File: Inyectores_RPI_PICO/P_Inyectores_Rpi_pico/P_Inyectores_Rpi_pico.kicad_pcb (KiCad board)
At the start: 2 copper layers, 127 x 139 mm, 98 parts, among them J1 Entrada_12V/4A, J2 Conn_01x07_Male, K1 SANYOU_SRD_Form_C, K2 SANYOU_SRD_Form_C, Q1 IRF540N, Q2 IRF540N, Q3 IRF540N, Q4 IRF540N, Q5 BC548, Q6 BC548, Q7 BC548, SW1 PUSH2, SW2 Reset_Push, SW3 Rotary_Encoder_Switch, SW4 PUSH1, U1 PC817, U10 DS3231M, U11 AT24CS32-XHM, U2 PC817, U3 PC817, U4 PC817, U5 L7805, U6 AMS1117-3.3, U7 Pico, U8 PC817, U9 PC817

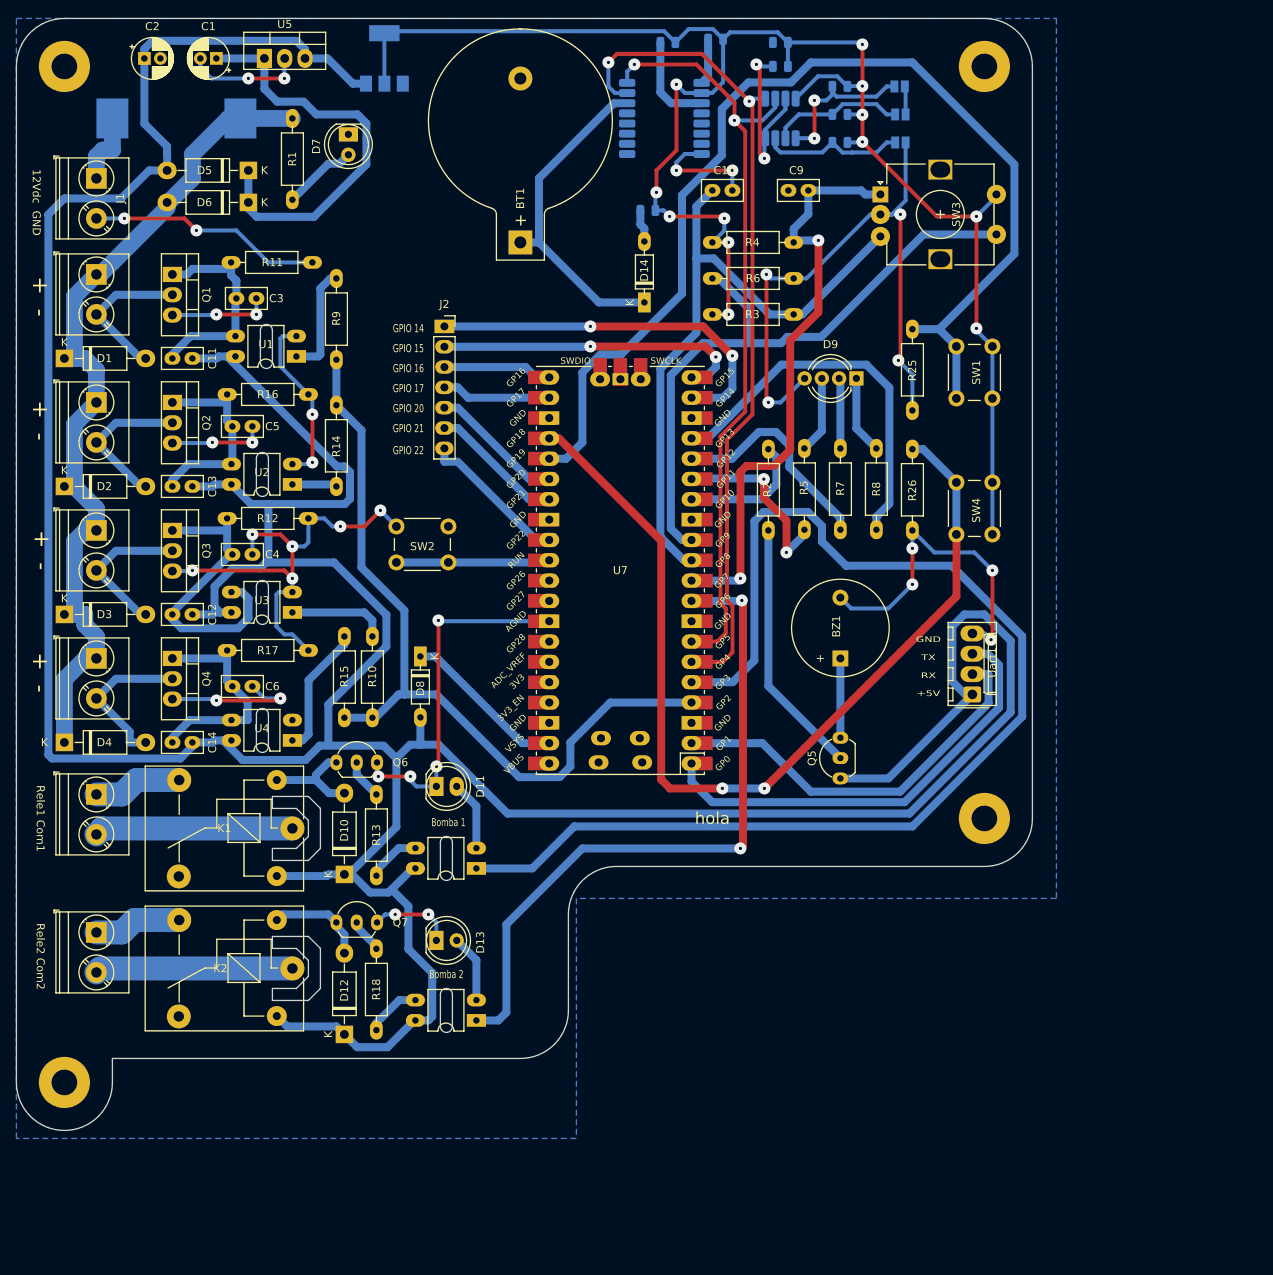
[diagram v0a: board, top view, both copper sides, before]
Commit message: Insoladora UV
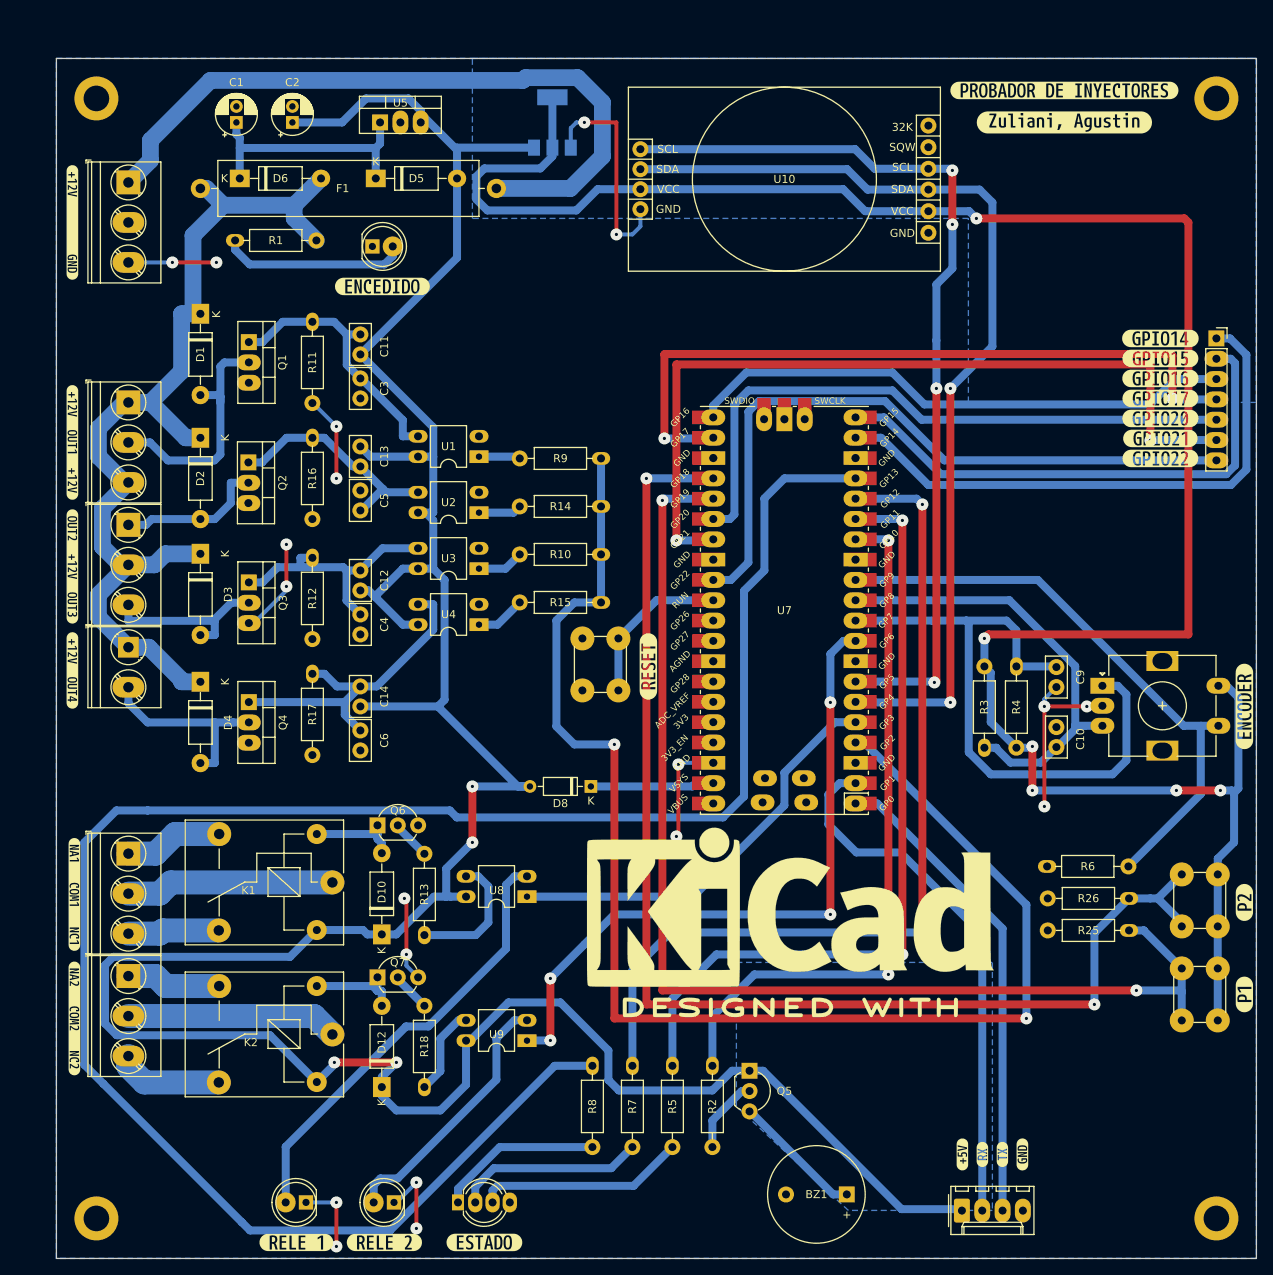
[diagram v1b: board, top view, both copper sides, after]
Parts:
- removed BT1: Battery_Cell, Battery:BatteryHolder_Keystone_103_1x20mm
- removed Bornera_rele1, Bornera_rele2, SAL_INY1, SAL_INY2, SAL_INY3: Screw_Terminal_01x02, Bornera_Tornillos:TerminalBlock_Phoenix_PT-1,5-2-5.0-H_1x02_P5.00mm_Horizontal
- removed C7, C8: 0.1uf, Capacitor_SMD:C_0805_2012Metric
- removed D14: 1N4148, Diode_THT:D_DO-35_SOD27_P7.62mm_Horizontal
- removed JP1: A0, Jumper:SolderJumper-2_P1.3mm_Open_Pad1.0x1.5mm
- removed JP2: A1, Jumper:SolderJumper-2_P1.3mm_Open_Pad1.0x1.5mm
- removed JP3: A2, Jumper:SolderJumper-2_P1.3mm_Open_Pad1.0x1.5mm
- removed R19: 200 1/8W 5%, Resistor_SMD:R_0805_2012Metric
- removed R20, R21: 4K7 1/8W 5%, Resistor_SMD:R_0805_2012Metric
- removed R22, R23, R24: 10k, Resistor_SMD:R_0805_2012Metric
- removed Tornillo1, Tornillo2, Tornillo3, Tornillo4: MountingHole_3.2mm_M3_Pad, MountingHole:MountingHole_3.2mm_M3_Pad
- removed U11: AT24CS32-XHM, Package_SO:SOIC-8_3.9x4.9mm_P1.27mm
- added ?: , , F.Cu at (170.0, 30.0)
- added J3: B1_INY, Borneras:TerminalBlock_Phoenix_PT-1,5-3-5.0-H_1x03_P5.00mm_Horizontal, F.Cu at (34.0, 68.0)
- added J4: BOR2_INY, Borneras:TerminalBlock_Phoenix_PT-1,5-3-5.0-H_1x03_P5.00mm_Horizontal, F.Cu at (34.0, 83.3)
- added J5: BOR1_RELE, Borneras:TerminalBlock_Phoenix_PT-1,5-3-5.0-H_1x03_P5.00mm_Horizontal, F.Cu at (34.0, 124.4)
- added J6: BOR2_RELE, Borneras:TerminalBlock_Phoenix_PT-1,5-3-5.0-H_1x03_P5.00mm_Horizontal, F.Cu at (34.0, 139.7)
- added REF3: MountingHole_3.2mm_M3_ISO14580_Pad, MountingHole:MountingHole_3.2mm_M3_ISO14580_Pad, F.Cu at (30.0, 170.0)
- added REF4: MountingHole_3.2mm_M3_ISO14580_Pad, MountingHole:MountingHole_3.2mm_M3_ISO14580_Pad, F.Cu at (170.0, 170.0)
- added REF5: MountingHole_3.2mm_M3_ISO14580_Pad, MountingHole:MountingHole_3.2mm_M3_ISO14580_Pad, F.Cu at (30.0, 30.0)
- added kibuzzard-62C09447: G***, kibuzzard-62C09447, F.Cu at (151.0, 33.0)
- added kibuzzard-62C09473: G***, kibuzzard-62C09473, F.Cu at (151.0, 29.0)
- added kibuzzard-62C095A2: G***, kibuzzard-62C095A2, F.Cu at (163.0, 60.0)
- added kibuzzard-62C095AC: G***, kibuzzard-62C095AC, F.Cu at (163.0, 62.5)
- added kibuzzard-62C095B6: G***, kibuzzard-62C095B6, F.Cu at (163.0, 65.0)
- added kibuzzard-62C095BF: G***, kibuzzard-62C095BF, F.Cu at (163.0, 67.5)
- added kibuzzard-62C095C6: G***, kibuzzard-62C095C6, F.Cu at (163.0, 70.0)
- added kibuzzard-62C095D0: G***, kibuzzard-62C095D0, F.Cu at (163.0, 72.5)
- added kibuzzard-62C095D9: G***, kibuzzard-62C095D9, F.Cu at (163.0, 75.0)
- added kibuzzard-62C09649: G***, kibuzzard-62C09649, F.Cu at (173.5, 142.0)
- added kibuzzard-62C09656: G***, kibuzzard-62C09656, F.Cu at (173.5, 130.5)
- added kibuzzard-62C09664: G***, kibuzzard-62C09664, F.Cu at (173.5, 106.0)
- added kibuzzard-62C0966F: G***, kibuzzard-62C0966F, F.Cu at (99.0, 101.0)
- added kibuzzard-62C096C0: G***, kibuzzard-62C096C0, F.Cu at (55.0, 173.0)
- added kibuzzard-62C096D5: G***, kibuzzard-62C096D5, F.Cu at (66.0, 173.0)
- added kibuzzard-62C096DE: G***, kibuzzard-62C096DE, F.Cu at (78.5, 173.0)
- added kibuzzard-62C096F9: G***, kibuzzard-62C096F9, F.Cu at (65.8, 53.5)
- added kibuzzard-62C09818: G***, kibuzzard-62C09818, F.Cu at (27.0, 88.5)
- added kibuzzard-62C09846: G***, kibuzzard-62C09846, F.Cu at (27.0, 101.5)
- added kibuzzard-62C098BB: G***, kibuzzard-62C098BB, F.Cu at (27.0, 73.0)
- added kibuzzard-62C09983: G***, kibuzzard-62C09983, F.Cu at (138.2, 162.0)
- added kibuzzard-62C099B8: G***, kibuzzard-62C099B8, F.Cu at (140.8, 162.0)
- added kibuzzard-62C099BF: G***, kibuzzard-62C099BF, F.Cu at (143.2, 162.0)
- added kibuzzard-62C099C8: G***, kibuzzard-62C099C8, F.Cu at (145.8, 162.0)
- added kibuzzard-62C099DD: G***, kibuzzard-62C099DD, F.Cu at (27.0, 45.5)
- added kibuzzard-62C09A4A: G***, kibuzzard-62C09A4A, F.Cu at (27.2, 129.5)
- added kibuzzard-62C09A65: G***, kibuzzard-62C09A65, F.Cu at (27.2, 145.0)
- F1: footprint Bornera_Tornillos:Fuse_20x5mm -> Fuse:Fuse_SunFuse-6HP; moved to F.Cu
- J1: footprint Bornera_Tornillos:TerminalBlock_Phoenix_PT-1,5-2-5.0-H_1x02_P5.00mm_Horizontal -> Borneras:TerminalBlock_Phoenix_PT-1,5-3-5.0-H_1x03_P5.00mm_Horizontal
- REF1: moved to F.Cu
- SAL_INY4: value Screw_Terminal_01x02 -> BOR3_INY; footprint Bornera_Tornillos:TerminalBlock_Phoenix_PT-1,5-2-5.0-H_1x02_P5.00mm_Horizontal -> Borneras:TerminalBlock_Phoenix_PT-1,5-2-5.0-H_1x02_P5.00mm_Horizontal
- U10: value DS3231M -> DS3231_SHIELD; footprint Package_SO:SOIC-16W_7.5x10.3mm_P1.27mm -> DS3231_SHIELD:DS3231_Shield; moved to F.Cu
- moved D9 114.4 mm to (75.2, 168.0), turned to 0 degrees
- moved J2 96.5 mm to (170.0, 60.0)
- moved R8 94.3 mm to (92.0, 161.1), turned to 90 degrees
- moved R7 91.1 mm to (97.0, 161.1), turned to 90 degrees
- moved R6 90.0 mm to (159.0, 126.0), turned to 180 degrees
- moved R5 88.9 mm to (102.0, 161.1), turned to 90 degrees
- moved SW1 82.7 mm to (170.2, 138.8)
- moved C10 81.8 mm to (150.0, 111.1), turned to 90 degrees
- moved R2 77.4 mm to (107.0, 161.1)
- moved R4 73.7 mm to (145.0, 111.2), turned to 90 degrees
- moved SW3 67.4 mm to (155.8, 103.4)
- moved R25 67.2 mm to (148.9, 134.0), turned to 0 degrees
- moved C9 67.2 mm to (150.0, 101.1), turned to -90 degrees
- moved BZ1 67.0 mm to (123.8, 167.0), turned to 180 degrees
- moved Uart1 64.5 mm to (138.2, 169.0), turned to 0 degrees
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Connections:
- net Net-(D1-Pad2) renamed /Control/INY1_OUT
- net Net-(D2-Pad2) renamed /Control/INY2_OUT
- net Net-(D3-Pad2) renamed /Control/INY3_OUT
- J1 pad 2: GND -> unconnected-(J1-Pad2)
- K1 pad 3: /Control/Sal_Rele1 -> /Control/Sal1_Rele1
- K1 pad 4: Net-(K1-Pad4) -> /Control/Sal2_Rele1
- K2 pad 3: /Control/Sal_Rele2 -> /Control/Sal1_Rele2
- K2 pad 4: Net-(K2-Pad4) -> /Control/Sal2_Rele2
- U10 pad 1: Net-(R20-Pad2) -> /Control/I2C0_SCL
- U10 pad 2: +3V3 -> /Control/I2C0_SDA
- U10 pad 3: Net-(R21-Pad2) -> +3V3
- U10 pad 4: Net-(U10-Pad4) -> GND
- U10 pad 5: GND -> unconnected-(U10-Pad5)
- U10 pad 6: GND -> unconnected-(U10-Pad6)
- U7 pad 13: Net-(U7-Pad13) -> unconnected-(U7-Pad13)
- U7 pad 18: Net-(U7-Pad18) -> unconnected-(U7-Pad18)
- U7 pad 23: Net-(U7-Pad23) -> unconnected-(U7-Pad23)
- U7 pad 28: Net-(U7-Pad28) -> unconnected-(U7-Pad28)
- U7 pad 3: Net-(U7-Pad3) -> unconnected-(U7-Pad3)
- U7 pad 31: Net-(U7-Pad31) -> unconnected-(U7-Pad31)
- U7 pad 32: Net-(U7-Pad32) -> unconnected-(U7-Pad32)
- U7 pad 34: Net-(U7-Pad34) -> unconnected-(U7-Pad34)
- U7 pad 35: Net-(U7-Pad35) -> unconnected-(U7-Pad35)
- U7 pad 36: Net-(U7-Pad36) -> unconnected-(U7-Pad36)
- U7 pad 37: Net-(U7-Pad37) -> unconnected-(U7-Pad37)
- U7 pad 40: Net-(U7-Pad40) -> unconnected-(U7-Pad40)
- U7 pad 41: Net-(U7-Pad41) -> unconnected-(U7-Pad41)
- U7 pad 42: Net-(U7-Pad42) -> unconnected-(U7-Pad42)
- U7 pad 43: Net-(U7-Pad43) -> unconnected-(U7-Pad43)
- U7 pad 8: Net-(U7-Pad8) -> unconnected-(U7-Pad8)
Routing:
- net GND: track 382.4 -> 127.7 mm, vias 36 -> 19
- net /Control/Rgb3: track 48.2 -> 244.7 mm
- net +5V: track 507.5 -> 391.2 mm, vias 0 -> 4
- net /Control/Bomba1: track 154.1 -> 52.5 mm
- net /Control/GPIO21: track 16.8 -> 103.7 mm, vias 0 -> 2
- net /Control/Rgb2: track 27.5 -> 112.5 mm, vias 0 -> 2
- net Net-(F1-Pad2): track 9.03 -> 89.1 mm
- net /Control/GPIO17: track 13.6 -> 91.2 mm, vias 0 -> 2
- net /Control/Rgb1: track 23.2 -> 99.6 mm
- net /Control/INYECTORES: track 99.9 -> 175.7 mm, vias 0 -> 2
- net /Control/Buzzer: track 16.2 -> 88.8 mm, vias 0 -> 2
- net +3V3: track 215.1 -> 283.2 mm, vias 12 -> 6
- net /Control/GPIO22: track 18.8 -> 86.3 mm
- net /Control/GPIO20: track 16.8 -> 79.1 mm
- net /Control/GPIO16: track 13.6 -> 69.1 mm
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- added copper zone on B.Cu, net +3V3
- added copper zone on B.Cu, net +5V
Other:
- board size 127 x 139 mm -> 150 x 150 mm
- board text removed: "+ -"
- board text removed: "12Vdc GND"
- board text removed: "Bomba 1"
- board text removed: "Bomba 2"
- board text removed: "GND TX RX +5V"
- board text removed: "GPIO 14"
- board text removed: "GPIO 15"
- board text removed: "GPIO 16"
- board text removed: "GPIO 17"
- board text removed: "GPIO 20"
- board text removed: "GPIO 21"
- board text removed: "GPIO 22"
- board text removed: "Rele1 Com1"
- board text removed: "Rele2 Com2"
- board text removed: "Zuliani, Agustin"
- board text removed: "hola"

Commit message: .
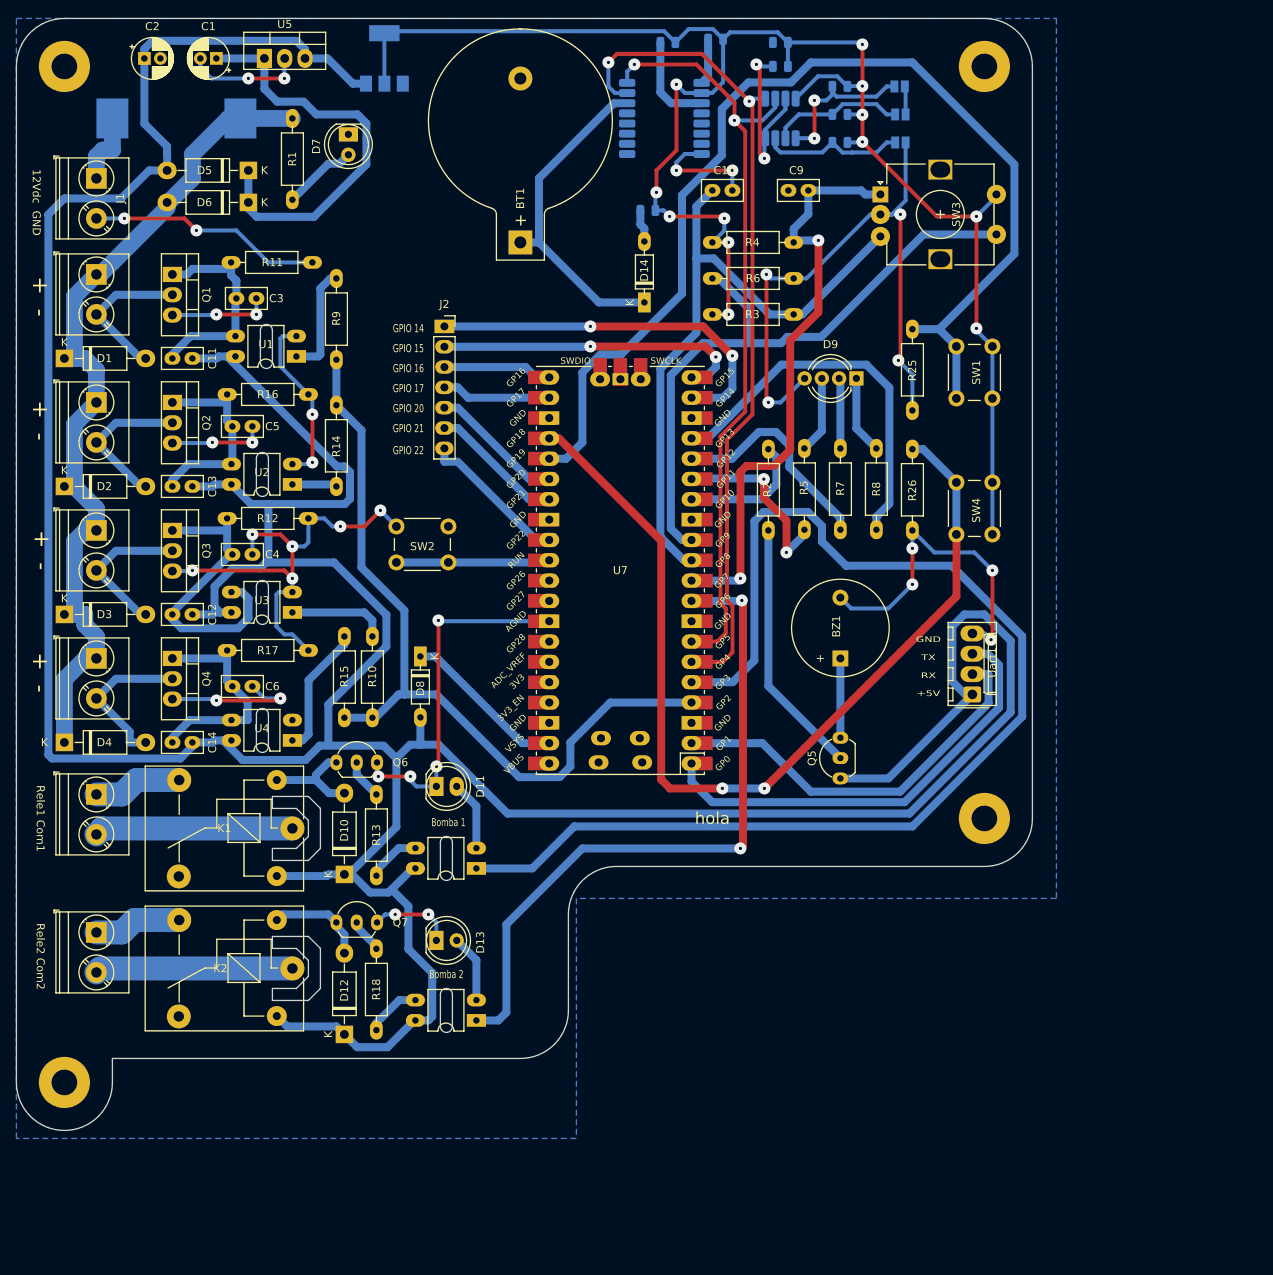
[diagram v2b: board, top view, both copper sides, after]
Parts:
- removed ?: , 
- removed J3: B1_INY, Borneras:TerminalBlock_Phoenix_PT-1,5-3-5.0-H_1x03_P5.00mm_Horizontal
- removed J4: BOR2_INY, Borneras:TerminalBlock_Phoenix_PT-1,5-3-5.0-H_1x03_P5.00mm_Horizontal
- removed J5: BOR1_RELE, Borneras:TerminalBlock_Phoenix_PT-1,5-3-5.0-H_1x03_P5.00mm_Horizontal
- removed J6: BOR2_RELE, Borneras:TerminalBlock_Phoenix_PT-1,5-3-5.0-H_1x03_P5.00mm_Horizontal
- removed REF3, REF4, REF5: MountingHole_3.2mm_M3_ISO14580_Pad, MountingHole:MountingHole_3.2mm_M3_ISO14580_Pad
- removed kibuzzard-62C09447: G***, kibuzzard-62C09447
- removed kibuzzard-62C09473: G***, kibuzzard-62C09473
- removed kibuzzard-62C095A2: G***, kibuzzard-62C095A2
- removed kibuzzard-62C095AC: G***, kibuzzard-62C095AC
- removed kibuzzard-62C095B6: G***, kibuzzard-62C095B6
- removed kibuzzard-62C095BF: G***, kibuzzard-62C095BF
- removed kibuzzard-62C095C6: G***, kibuzzard-62C095C6
- removed kibuzzard-62C095D0: G***, kibuzzard-62C095D0
- removed kibuzzard-62C095D9: G***, kibuzzard-62C095D9
- removed kibuzzard-62C09649: G***, kibuzzard-62C09649
- removed kibuzzard-62C09656: G***, kibuzzard-62C09656
- removed kibuzzard-62C09664: G***, kibuzzard-62C09664
- removed kibuzzard-62C0966F: G***, kibuzzard-62C0966F
- removed kibuzzard-62C096C0: G***, kibuzzard-62C096C0
- removed kibuzzard-62C096D5: G***, kibuzzard-62C096D5
- removed kibuzzard-62C096DE: G***, kibuzzard-62C096DE
- removed kibuzzard-62C096F9: G***, kibuzzard-62C096F9
- removed kibuzzard-62C09818: G***, kibuzzard-62C09818
- removed kibuzzard-62C09846: G***, kibuzzard-62C09846
- removed kibuzzard-62C098BB: G***, kibuzzard-62C098BB
- removed kibuzzard-62C09983: G***, kibuzzard-62C09983
- removed kibuzzard-62C099B8: G***, kibuzzard-62C099B8
- removed kibuzzard-62C099BF: G***, kibuzzard-62C099BF
- removed kibuzzard-62C099C8: G***, kibuzzard-62C099C8
- removed kibuzzard-62C099DD: G***, kibuzzard-62C099DD
- removed kibuzzard-62C09A4A: G***, kibuzzard-62C09A4A
- removed kibuzzard-62C09A65: G***, kibuzzard-62C09A65
- added BT1: Battery_Cell, Battery:BatteryHolder_Keystone_103_1x20mm, F.Cu at (83.0, 48.0)
- added Bornera_rele1: Screw_Terminal_01x02, Bornera_Tornillos:TerminalBlock_Phoenix_PT-1,5-2-5.0-H_1x02_P5.00mm_Horizontal, F.Cu at (30.0, 117.0)
- added Bornera_rele2: Screw_Terminal_01x02, Bornera_Tornillos:TerminalBlock_Phoenix_PT-1,5-2-5.0-H_1x02_P5.00mm_Horizontal, F.Cu at (30.0, 134.2)
- added C7: 0.1uf, Capacitor_SMD:C_0805_2012Metric, B.Cu at (115.5, 26.0)
- added C8: 0.1uf, Capacitor_SMD:C_0805_2012Metric, B.Cu at (115.5, 23.0)
- added D14: 1N4148, Diode_THT:D_DO-35_SOD27_P7.62mm_Horizontal, F.Cu at (98.5, 55.5)
- added JP1: A0, Jumper:SolderJumper-2_P1.3mm_Open_Pad1.0x1.5mm, B.Cu at (130.4, 28.5)
- added JP2: A1, Jumper:SolderJumper-2_P1.3mm_Open_Pad1.0x1.5mm, B.Cu at (130.5, 32.0)
- added JP3: A2, Jumper:SolderJumper-2_P1.3mm_Open_Pad1.0x1.5mm, B.Cu at (130.5, 35.5)
- added R19: 200 1/8W 5%, Resistor_SMD:R_0805_2012Metric, B.Cu at (98.9, 44.0)
- added R20: 4K7 1/8W 5%, Resistor_SMD:R_0805_2012Metric, B.Cu at (107.4, 22.6)
- added R21: 4K7 1/8W 5%, Resistor_SMD:R_0805_2012Metric, B.Cu at (101.4, 23.0)
- added R22: 10k, Resistor_SMD:R_0805_2012Metric, B.Cu at (122.9, 35.5)
- added R23: 10k, Resistor_SMD:R_0805_2012Metric, B.Cu at (122.9, 32.0)
- added R24: 10k, Resistor_SMD:R_0805_2012Metric, B.Cu at (122.9, 28.5)
- added SAL_INY1: Screw_Terminal_01x02, Bornera_Tornillos:TerminalBlock_Phoenix_PT-1,5-2-5.0-H_1x02_P5.00mm_Horizontal, F.Cu at (30.0, 52.0)
- added SAL_INY2: Screw_Terminal_01x02, Bornera_Tornillos:TerminalBlock_Phoenix_PT-1,5-2-5.0-H_1x02_P5.00mm_Horizontal, F.Cu at (30.0, 68.0)
- added SAL_INY3: Screw_Terminal_01x02, Bornera_Tornillos:TerminalBlock_Phoenix_PT-1,5-2-5.0-H_1x02_P5.00mm_Horizontal, F.Cu at (30.0, 84.0)
- added Tornillo1: MountingHole_3.2mm_M3_Pad, MountingHole:MountingHole_3.2mm_M3_Pad, F.Cu at (141.0, 120.0)
- added Tornillo2: MountingHole_3.2mm_M3_Pad, MountingHole:MountingHole_3.2mm_M3_Pad, F.Cu at (26.0, 26.0)
- added Tornillo3: MountingHole_3.2mm_M3_Pad, MountingHole:MountingHole_3.2mm_M3_Pad, F.Cu at (26.0, 153.0)
- added Tornillo4: MountingHole_3.2mm_M3_Pad, MountingHole:MountingHole_3.2mm_M3_Pad, F.Cu at (141.0, 26.0)
- added U11: AT24CS32-XHM, Package_SO:SOIC-8_3.9x4.9mm_P1.27mm, B.Cu at (115.5, 32.5)
- F1: footprint Fuse:Fuse_SunFuse-6HP -> Bornera_Tornillos:Fuse_20x5mm; moved to B.Cu
- J1: footprint Borneras:TerminalBlock_Phoenix_PT-1,5-3-5.0-H_1x03_P5.00mm_Horizontal -> Bornera_Tornillos:TerminalBlock_Phoenix_PT-1,5-2-5.0-H_1x02_P5.00mm_Horizontal
- REF1: moved to B.Cu
- SAL_INY4: value BOR3_INY -> Screw_Terminal_01x02; footprint Borneras:TerminalBlock_Phoenix_PT-1,5-2-5.0-H_1x02_P5.00mm_Horizontal -> Bornera_Tornillos:TerminalBlock_Phoenix_PT-1,5-2-5.0-H_1x02_P5.00mm_Horizontal
- U10: value DS3231_SHIELD -> DS3231M; footprint DS3231_SHIELD:DS3231_Shield -> Package_SO:SOIC-16W_7.5x10.3mm_P1.27mm; moved to B.Cu
- moved D9 114.4 mm to (125.0, 65.0), turned to 180 degrees
- moved J2 96.5 mm to (73.5, 58.5)
- moved R8 94.3 mm to (127.5, 73.8), turned to -90 degrees
- moved R7 91.1 mm to (123.0, 73.8), turned to -90 degrees
- moved R6 90.0 mm to (107.0, 52.5), turned to 0 degrees
- moved R5 88.9 mm to (118.5, 73.8), turned to -90 degrees
- moved SW1 82.7 mm to (142.0, 61.0)
- moved C10 81.8 mm to (107.0, 41.5), turned to 0 degrees
- moved R2 77.4 mm to (114.0, 84.0)
- moved R4 73.7 mm to (107.0, 48.0), turned to 0 degrees
- moved SW3 67.4 mm to (128.0, 42.0)
- moved R25 67.2 mm to (132.0, 69.0), turned to 90 degrees
- moved C9 67.2 mm to (119.0, 41.5), turned to 180 degrees
- moved BZ1 67.0 mm to (123.0, 100.0), turned to 90 degrees
- moved Uart1 64.5 mm to (139.5, 104.5), turned to 90 degrees
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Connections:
- net /Control/INY1_OUT renamed Net-(D1-Pad2)
- net /Control/INY2_OUT renamed Net-(D2-Pad2)
- net /Control/INY3_OUT renamed Net-(D3-Pad2)
- J1 pad 2: unconnected-(J1-Pad2) -> GND
- K1 pad 3: /Control/Sal1_Rele1 -> /Control/Sal_Rele1
- K1 pad 4: /Control/Sal2_Rele1 -> Net-(K1-Pad4)
- K2 pad 3: /Control/Sal1_Rele2 -> /Control/Sal_Rele2
- K2 pad 4: /Control/Sal2_Rele2 -> Net-(K2-Pad4)
- U10 pad 1: /Control/I2C0_SCL -> Net-(R20-Pad2)
- U10 pad 2: /Control/I2C0_SDA -> +3V3
- U10 pad 3: +3V3 -> Net-(R21-Pad2)
- U10 pad 4: GND -> Net-(U10-Pad4)
- U10 pad 5: unconnected-(U10-Pad5) -> GND
- U10 pad 6: unconnected-(U10-Pad6) -> GND
- U7 pad 13: unconnected-(U7-Pad13) -> Net-(U7-Pad13)
- U7 pad 18: unconnected-(U7-Pad18) -> Net-(U7-Pad18)
- U7 pad 23: unconnected-(U7-Pad23) -> Net-(U7-Pad23)
- U7 pad 28: unconnected-(U7-Pad28) -> Net-(U7-Pad28)
- U7 pad 3: unconnected-(U7-Pad3) -> Net-(U7-Pad3)
- U7 pad 31: unconnected-(U7-Pad31) -> Net-(U7-Pad31)
- U7 pad 32: unconnected-(U7-Pad32) -> Net-(U7-Pad32)
- U7 pad 34: unconnected-(U7-Pad34) -> Net-(U7-Pad34)
- U7 pad 35: unconnected-(U7-Pad35) -> Net-(U7-Pad35)
- U7 pad 36: unconnected-(U7-Pad36) -> Net-(U7-Pad36)
- U7 pad 37: unconnected-(U7-Pad37) -> Net-(U7-Pad37)
- U7 pad 40: unconnected-(U7-Pad40) -> Net-(U7-Pad40)
- U7 pad 41: unconnected-(U7-Pad41) -> Net-(U7-Pad41)
- U7 pad 42: unconnected-(U7-Pad42) -> Net-(U7-Pad42)
- U7 pad 43: unconnected-(U7-Pad43) -> Net-(U7-Pad43)
- U7 pad 8: unconnected-(U7-Pad8) -> Net-(U7-Pad8)
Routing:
- net GND: track 127.7 -> 382.4 mm, vias 19 -> 36
- net /Control/Rgb3: track 244.7 -> 48.2 mm
- net +5V: track 391.2 -> 507.5 mm, vias 4 -> 0
- net /Control/Bomba1: track 52.5 -> 154.1 mm
- net /Control/GPIO21: track 103.7 -> 16.8 mm, vias 2 -> 0
- net /Control/Rgb2: track 112.5 -> 27.5 mm, vias 2 -> 0
- net Net-(F1-Pad2): track 89.1 -> 9.03 mm
- net /Control/GPIO17: track 91.2 -> 13.6 mm, vias 2 -> 0
- net /Control/Rgb1: track 99.6 -> 23.2 mm
- net /Control/INYECTORES: track 175.7 -> 99.9 mm, vias 2 -> 0
- net /Control/Buzzer: track 88.8 -> 16.2 mm, vias 2 -> 0
- net +3V3: track 283.2 -> 215.1 mm, vias 6 -> 12
- net /Control/GPIO22: track 86.3 -> 18.8 mm
- net /Control/GPIO20: track 79.1 -> 16.8 mm
- net /Control/GPIO16: track 69.1 -> 13.6 mm
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- removed copper zone on B.Cu, net +3V3
- removed copper zone on B.Cu, net +5V
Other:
- board size 150 x 150 mm -> 127 x 139 mm
- board text added: "+ -"
- board text added: "12Vdc GND"
- board text added: "Bomba 1"
- board text added: "Bomba 2"
- board text added: "GND TX RX +5V"
- board text added: "GPIO 14"
- board text added: "GPIO 15"
- board text added: "GPIO 16"
- board text added: "GPIO 17"
- board text added: "GPIO 20"
- board text added: "GPIO 21"
- board text added: "GPIO 22"
- board text added: "Rele1 Com1"
- board text added: "Rele2 Com2"
- board text added: "Zuliani, Agustin"
- board text added: "hola"
